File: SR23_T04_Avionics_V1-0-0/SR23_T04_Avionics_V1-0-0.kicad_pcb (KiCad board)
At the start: 2 copper layers, 50 parts, among them J1 QWIIC, J11 Conn_01x02, J12 Conn_01x02, J13 Conn_01x02, J14 BAT_CHARGE, J2 QWIIC, J3 QWIIC, J4 BAT_POWER, J5 BAT_uC, J6 BAT_PCB+, J7 Conn_01x03, J8 Conn_01x03, J9 Conn_01x03, Q2 BSP75N, Q3 BSP75N, Q4 BSP75N, SW1 SW_DIP_x02, U1 MCP73831-2-OT, U2 MS563702BA03-50, U3 MPU-6050, U4 MOUDLE-SEEEDUINO-XIAO-ESP32C3

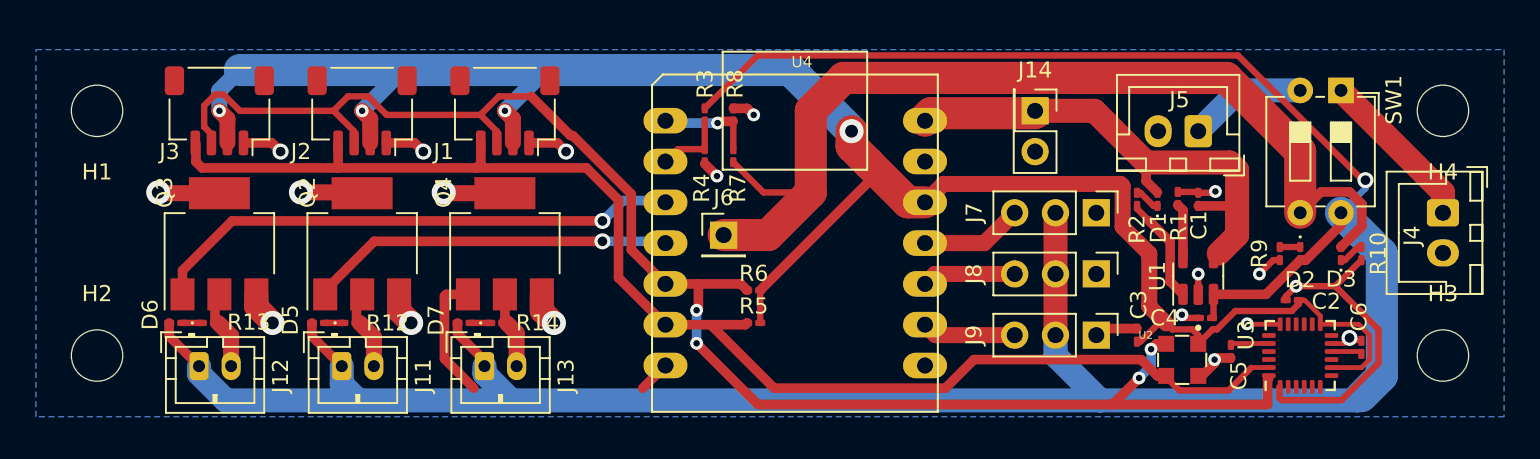
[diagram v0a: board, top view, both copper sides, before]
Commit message: feat: Version 1.0.0 of the AV-Flow PCB
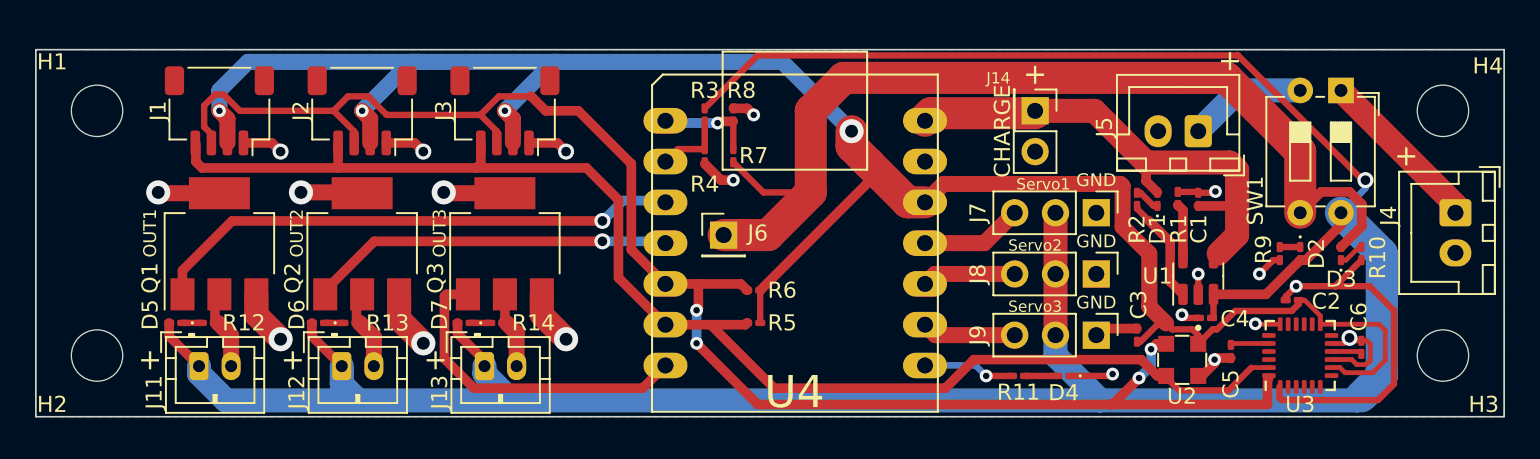
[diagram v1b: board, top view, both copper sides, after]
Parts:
- added D4: GREEN, LED_SMD:LED_0201_0603Metric_Pad0.64x0.40mm_HandSolder, F.Cu at (161.8, 108.0)
- added R11: 540, Resistor_SMD:R_0201_0603Metric_Pad0.64x0.40mm_HandSolder, F.Cu at (159.0, 108.0)
- moved J4 0.78 mm to (186.2, 97.8)
- renumbered D6 to D5, D5 to D6, J3 to J1, J12 to J11, J11 to J12, J1 to J3, Q3 to Q1, Q4 to Q3, R13 to R12, R12 to R13
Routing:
- net GND: track 63.7 -> 78.8 mm, vias 19 -> 20
- net OUT3: track 10.0 -> 20.5 mm
- net OUT4: track 0.00 -> 5.69 mm, vias 0 -> 1
- net +3.3V: track 121.1 -> 126.1 mm
- net Net-(D4-Pad2): track 0.00 -> 2.00 mm
- net SDA: track 98.4 -> 99.5 mm
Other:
- board outline added: 91.4 x 22.9 mm
- board text added: "+"
- board text added: "CHARGE"
- board text added: "GND"
- board text added: "OUT1"
- board text added: "OUT2"
- board text added: "OUT3"
- board text added: "Project: AV-Flow Version: 1.0.0 Date: 11.04.2023 Author: Florian Patiny Co-author: Luc Patiny"
- board text added: "Servo1"
- board text added: "Servo2"
- board text added: "Servo3"

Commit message: wip: PCB V2
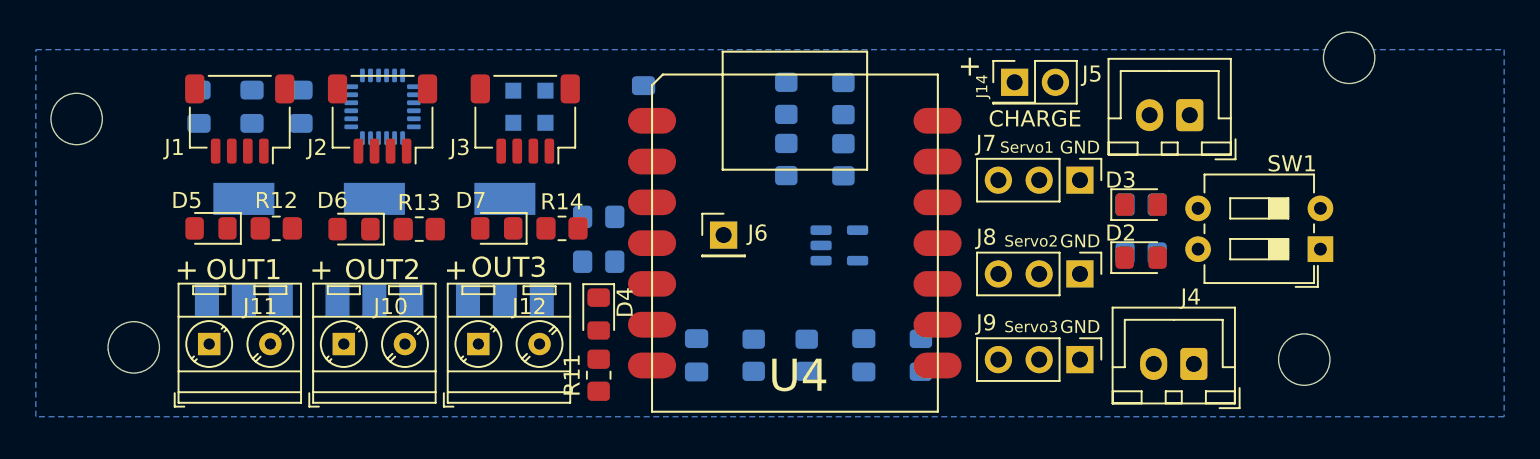
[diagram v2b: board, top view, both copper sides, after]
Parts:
- removed J13: Conn_01x02, Connector_JST:JST_PH_B2B-PH-K_1x02_P2.00mm_Vertical
- added J10: Screw_Terminal_01x02, TerminalBlock_MetzConnect:TerminalBlock_MetzConnect_Type086_RT03402HBLC_1x02_P3.81mm_Horizontal, F.Cu at (117.0, 106.0)
- C1, C2, C3, C4, C5, C6: footprint Capacitor_SMD:C_0201_0603Metric_Pad0.64x0.40mm_HandSolder -> Capacitor_SMD:C_0805_2012Metric_Pad1.18x1.45mm_HandSolder; moved to B.Cu
- D1: footprint LED_SMD:LED_0201_0603Metric_Pad0.64x0.40mm_HandSolder -> LED_SMD:LED_0805_2012Metric_Pad1.15x1.40mm_HandSolder; moved to B.Cu
- D2, D3, D5, D6, D7: footprint LED_SMD:LED_0201_0603Metric_Pad0.64x0.40mm_HandSolder -> LED_SMD:LED_0805_2012Metric_Pad1.15x1.40mm_HandSolder
- D4: value GREEN -> LED; footprint LED_SMD:LED_0201_0603Metric_Pad0.64x0.40mm_HandSolder -> LED_SMD:LED_0805_2012Metric_Pad1.15x1.40mm_HandSolder
- J11, J12: value Conn_01x02 -> Screw_Terminal_01x02; footprint Connector_JST:JST_PH_B2B-PH-K_1x02_P2.00mm_Vertical -> TerminalBlock_MetzConnect:TerminalBlock_MetzConnect_Type086_RT03402HBLC_1x02_P3.81mm_Horizontal
- Q1, Q2, Q3, U1, U2, U3: moved to B.Cu
- R1, R10, R2, R3, R4, R5, R6, R7, R8, R9: footprint Resistor_SMD:R_0201_0603Metric_Pad0.64x0.40mm_HandSolder -> Resistor_SMD:R_0805_2012Metric_Pad1.20x1.40mm_HandSolder; moved to B.Cu
- R11, R12, R13, R14: footprint Resistor_SMD:R_0201_0603Metric_Pad0.64x0.40mm_HandSolder -> Resistor_SMD:R_0805_2012Metric_Pad1.20x1.40mm_HandSolder
- moved C6 67.7 mm to (114.3, 91.2)
- moved C5 66.0 mm to (108.0, 91.2)
- moved C2 65.9 mm to (111.3, 91.2), turned to -90 degrees
- moved U3 59.2 mm to (119.4, 91.2), turned to 180 degrees
- moved U2 43.6 mm to (128.5, 91.2)
- moved C3 34.0 mm to (135.6, 90.9)
- moved C4 31.8 mm to (138.9, 106.7), turned to -90 degrees
- moved D4 29.2 mm to (132.8, 104.1), turned to -90 degrees
- moved R11 26.1 mm to (132.8, 107.9), turned to 90 degrees
- moved R2 25.8 mm to (142.5, 106.7)
- moved R1 25.1 mm to (145.8, 106.7)
- moved C1 23.0 mm to (149.4, 106.7)
- moved U1 22.4 mm to (147.8, 99.8), turned to 0 degrees
- moved H3 19.4 mm to (179.6, 88.1)
- moved J4 18.8 mm to (169.9, 107.2), turned to 180 degrees
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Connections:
- J12 pad 2: Net-(J12-Pad2) -> Net-(Q3-Pad2)
- Q2 pad 2: Net-(J12-Pad2) -> Net-(Q2-Pad2)
- Q3 pad 1: OUT3 -> OUT4
- Q3 pad 2: Net-(J13-Pad2) -> Net-(Q3-Pad2)
- R11 pad 1: OUT4 -> OUT3
- R13 pad 2: Net-(J12-Pad2) -> Net-(Q2-Pad2)
- R14 pad 2: Net-(J13-Pad2) -> Net-(Q3-Pad2)
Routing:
- net DIP_1b: track 175.5 -> 0.00 mm, vias 1 -> 0
- net +3.3V: track 126.1 -> 0.00 mm, vias 4 -> 0
- net SDA: track 99.5 -> 0.00 mm, vias 4 -> 0
- net SCL: track 84.6 -> 0.00 mm
- net GND: track 78.8 -> 0.00 mm, vias 20 -> 0
- net DIP_2b: track 62.2 -> 0.00 mm
- net OUT1: track 33.4 -> 0.00 mm, vias 1 -> 0
- net VUSB: track 31.6 -> 0.00 mm
- net OUT2: track 22.7 -> 0.00 mm, vias 1 -> 0
- net OUT3: track 20.5 -> 0.00 mm
- net DIP_1a: track 10.6 -> 0.00 mm
- net DIP_2a: track 7.40 -> 0.00 mm
- net STAT: track 6.69 -> 0.00 mm
- net Servo1: track 6.37 -> 0.00 mm
- net MON_BAT_uC: track 6.05 -> 0.00 mm, vias 1 -> 0
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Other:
- board outline removed
